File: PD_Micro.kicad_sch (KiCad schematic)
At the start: 55 parts, among them J1 Conn_01x02, J2 Conn_01x02, J3 USB_C_Receptacle_USB2.0, J4 Conn_01x02, J5 Conn_01x02, J7 Conn_01x02, J8 Conn_01x02, Q1 BC847, Q4 IRF9393, SW1 SW_DIP_x06, SW2 SW_DPST_x2, SW3 SW_Push, SW4 SW_Push, SW5 SW_DPST_x2, U1 SRV05-4, U2 Pico, U3 TMCS1108, U6 oledSym, U7 LMR54410

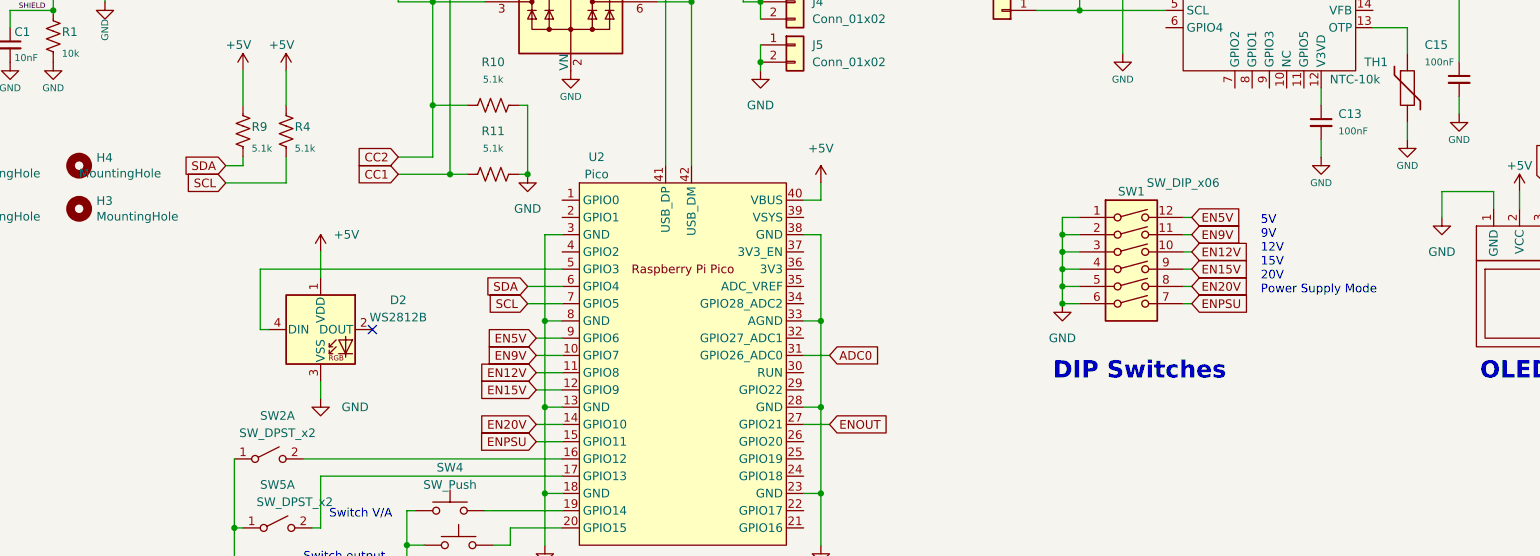
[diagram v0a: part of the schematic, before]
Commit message: finished
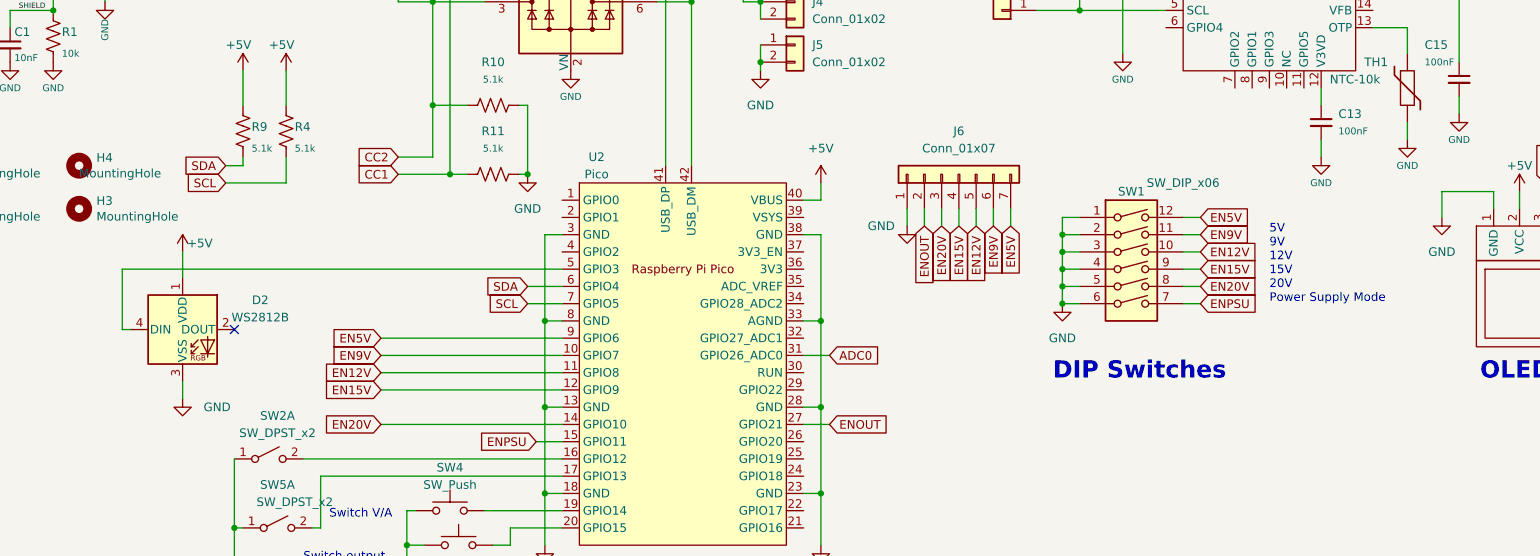
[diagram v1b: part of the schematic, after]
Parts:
- added J6: Conn_01x07, Connector_PinSocket_2.54mm:PinSocket_1x07_P2.54mm_Vertical, symbol Connector_Generic:Conn_01x07
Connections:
- net EN12V: now also J6.5 (Pin_5)
- net EN15V: now also J6.4 (Pin_4)
- net EN20V: now also J6.3 (Pin_3)
- net EN5V: now also J6.7 (Pin_7)
- net EN9V: now also J6.6 (Pin_6)
- net ENOUT: now also J6.2 (Pin_2)
- net GND: now also J6.1 (Pin_1)
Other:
- moved on the sheet: D2

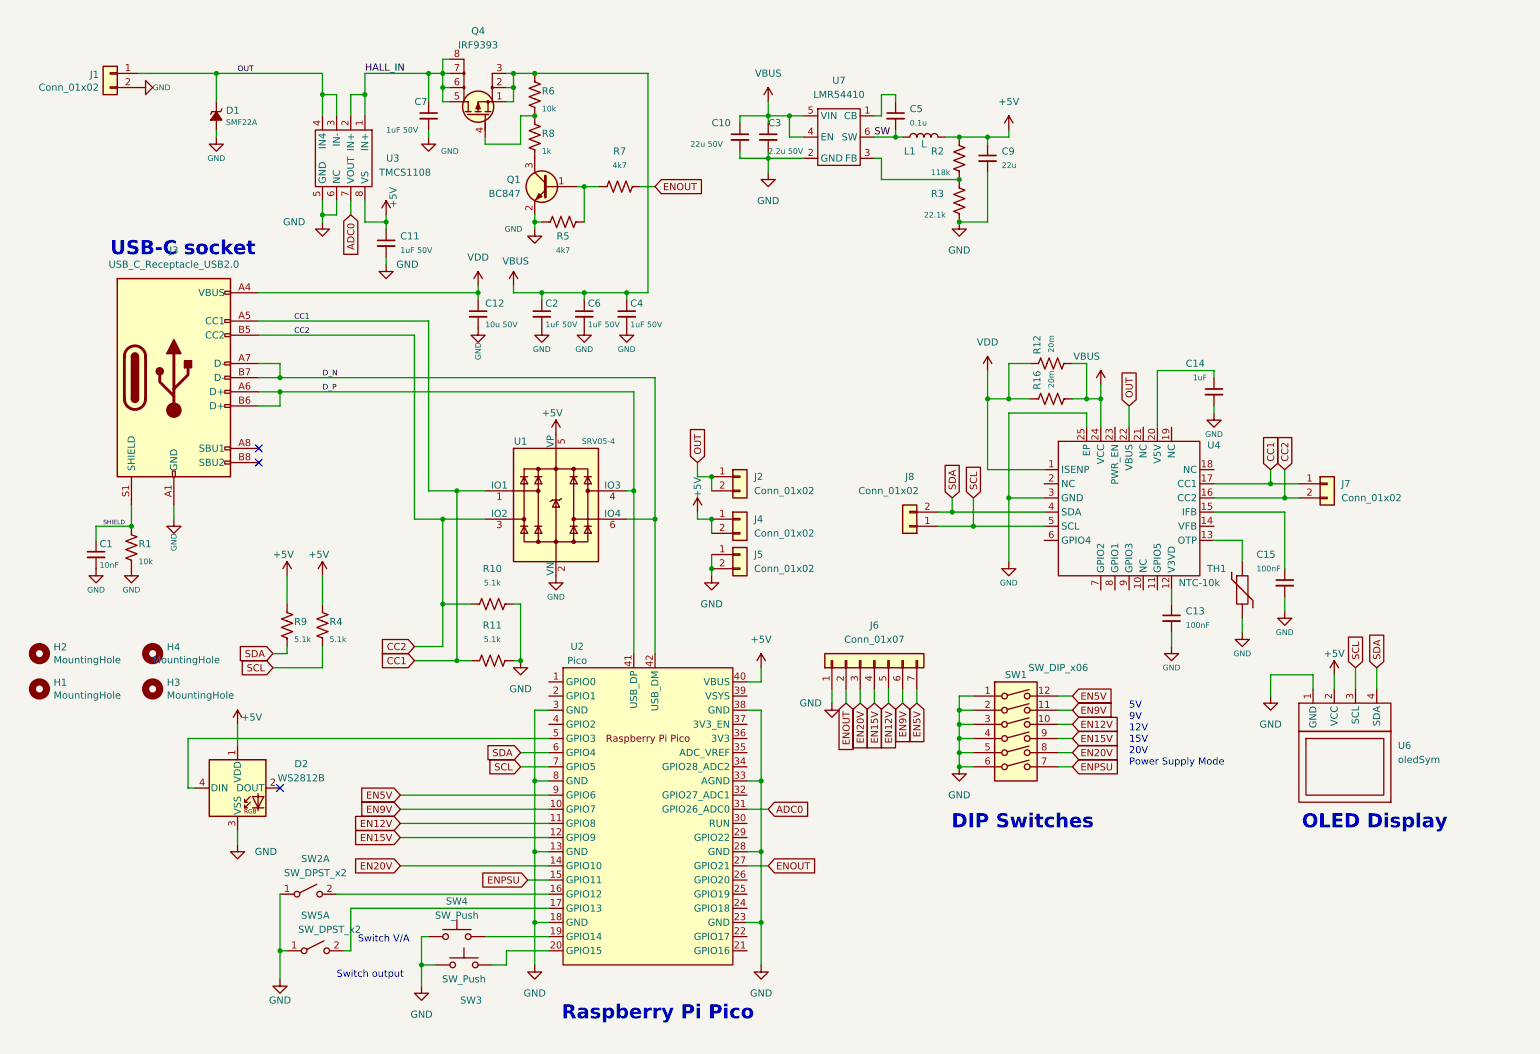
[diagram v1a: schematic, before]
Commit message: final
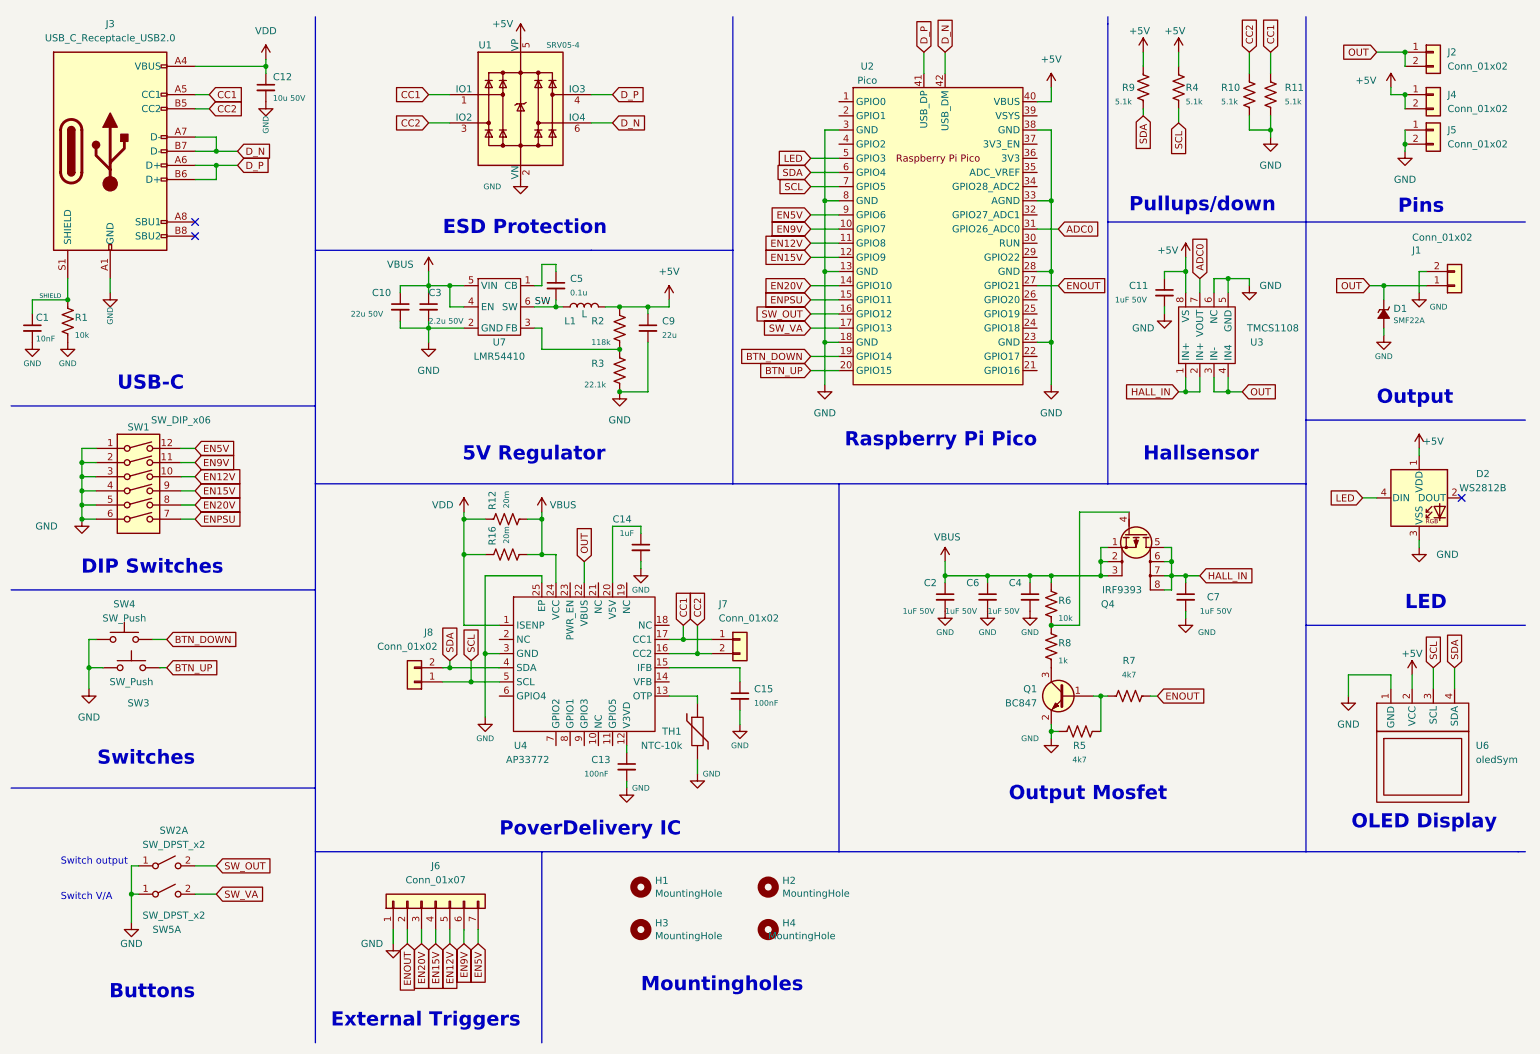
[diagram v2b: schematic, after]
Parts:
- U4: value ~ -> AP33772
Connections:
- net SW_OUT: now reaches SW2.2 (B), U2.16 (GPIO12)
- net SW_VA: now reaches SW5.2 (B), U2.17 (GPIO13)
- net BTN_DOWN: now reaches SW4.2, U2.19 (GPIO14)
- net BTN_UP: now reaches SW3.2, U2.20 (GPIO15)
- net LED: now reaches D2.4 (DIN), U2.5 (GPIO3)
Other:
- note added: "5V Regulator"
- note added: "Buttons"
- note added: "ESD Protection"
- note added: "External Triggers"
- note added: "Hallsensor"
- note added: "LED"
- note added: "Mountingholes"
- note added: "Output"
- note added: "Output Mosfet"
- note added: "Pins"
- note added: "PoverDelivery IC"
- note added: "Pullups/down"
- note added: "Switches"
- note added: "USB-C"
- note removed: "5V 9V 12V 15V 20V Power Supply Mode"
- note removed: "USB-C socket"
- company: (none) -> HTL Rankweil
- title: (none) -> USBC_PD-Trigger
- moved on the sheet: C1, C10, C11, C12, C13, C14, C15, C2, C3, C4, C5, C6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
